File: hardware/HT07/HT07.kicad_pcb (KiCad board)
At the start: 2 copper layers, 54 x 54 mm, 35 parts, among them J30 Conn_02x04_Odd_Even, P1 Conn_01x01_MountingPin, P2 Conn_01x01_MountingPin, P3 Conn_01x01_MountingPin, P4 Conn_01x01_MountingPin, SW30 SW_Push, U1 HDC2021, U2 NT3H2111W0FTTJ, U3 MSP430FR2155TDBT, U4 SIP32431DR3-T1GE3, Y1 32K768

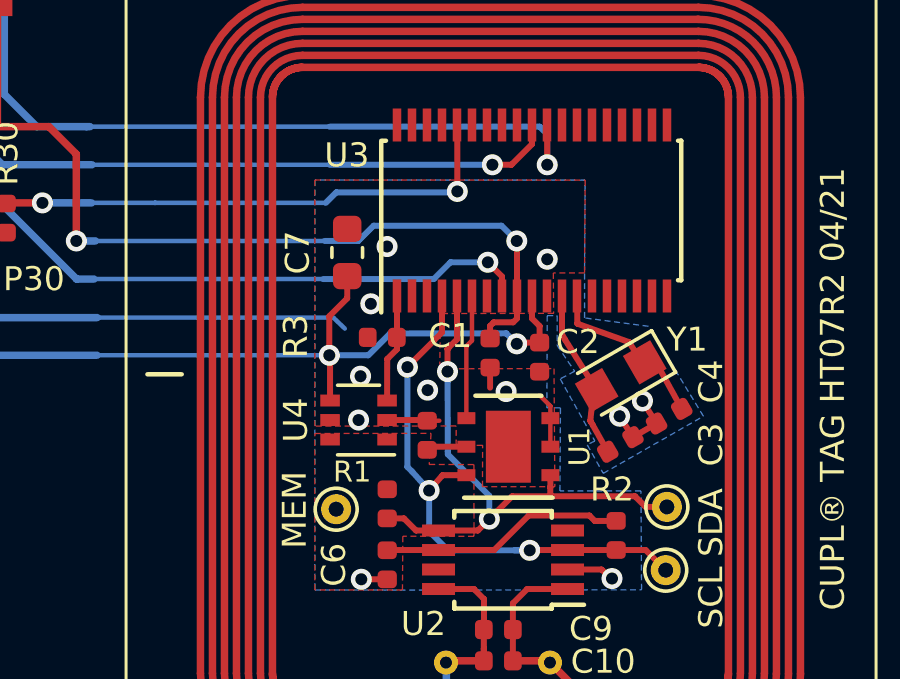
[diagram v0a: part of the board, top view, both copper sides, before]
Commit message: HT07R2 sent to manufacture at Eurocircuits
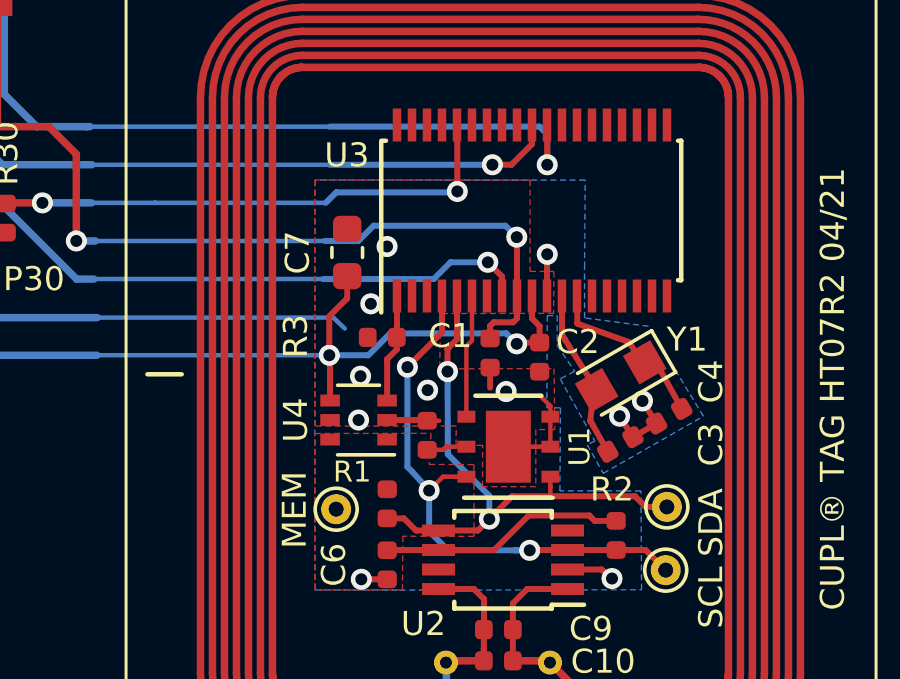
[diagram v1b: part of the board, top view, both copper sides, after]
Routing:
- net GND: track 30.6 -> 33.4 mm
